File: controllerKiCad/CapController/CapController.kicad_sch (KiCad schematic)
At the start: 16 parts

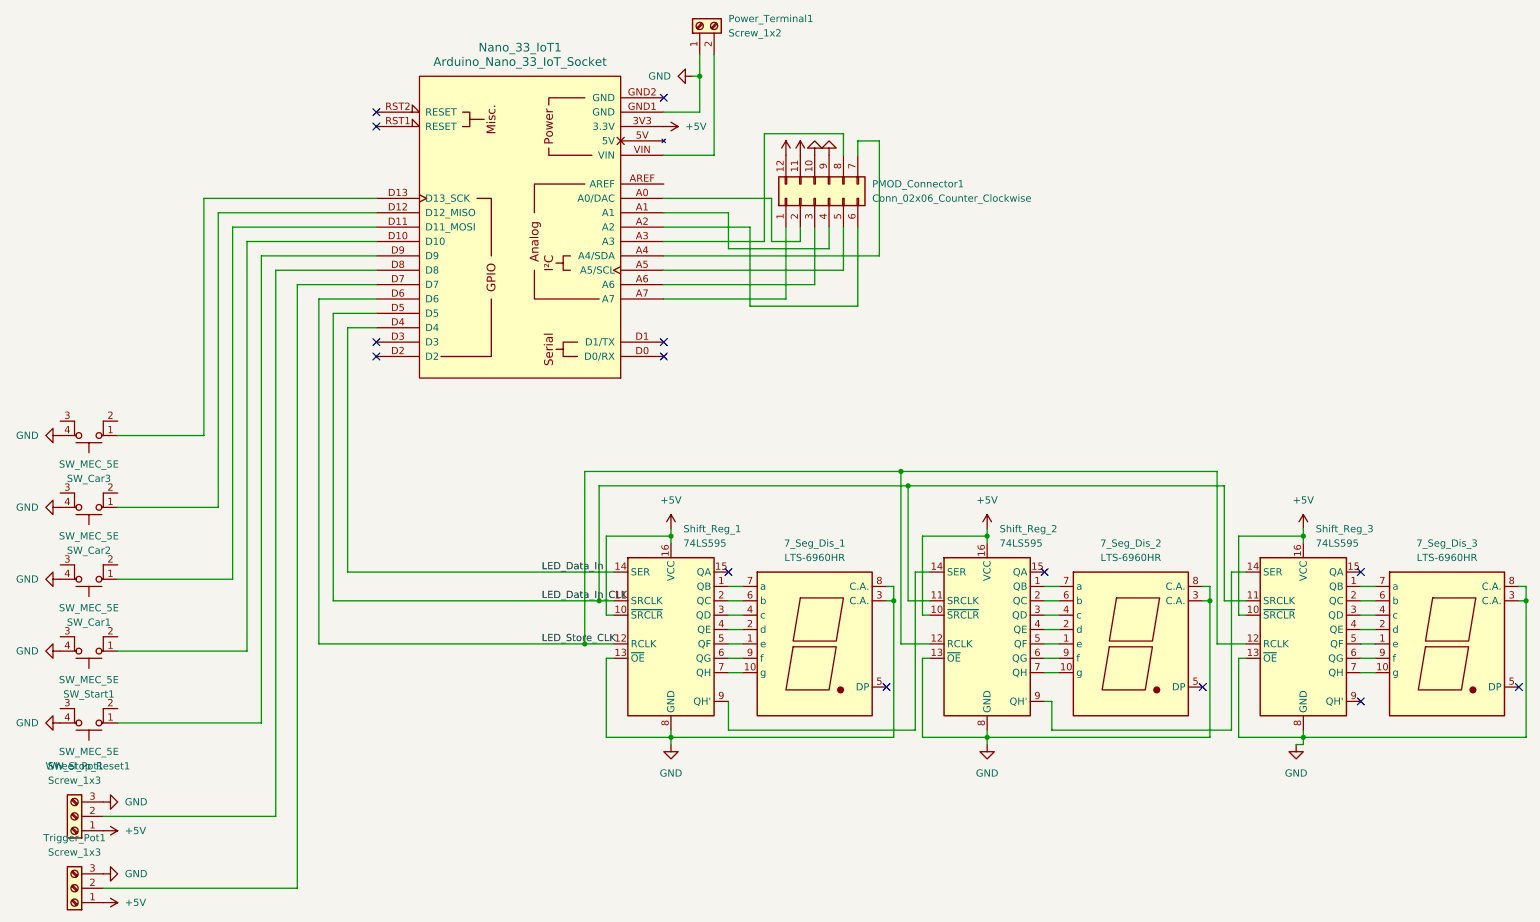
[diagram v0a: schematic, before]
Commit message: updated controller kicad files
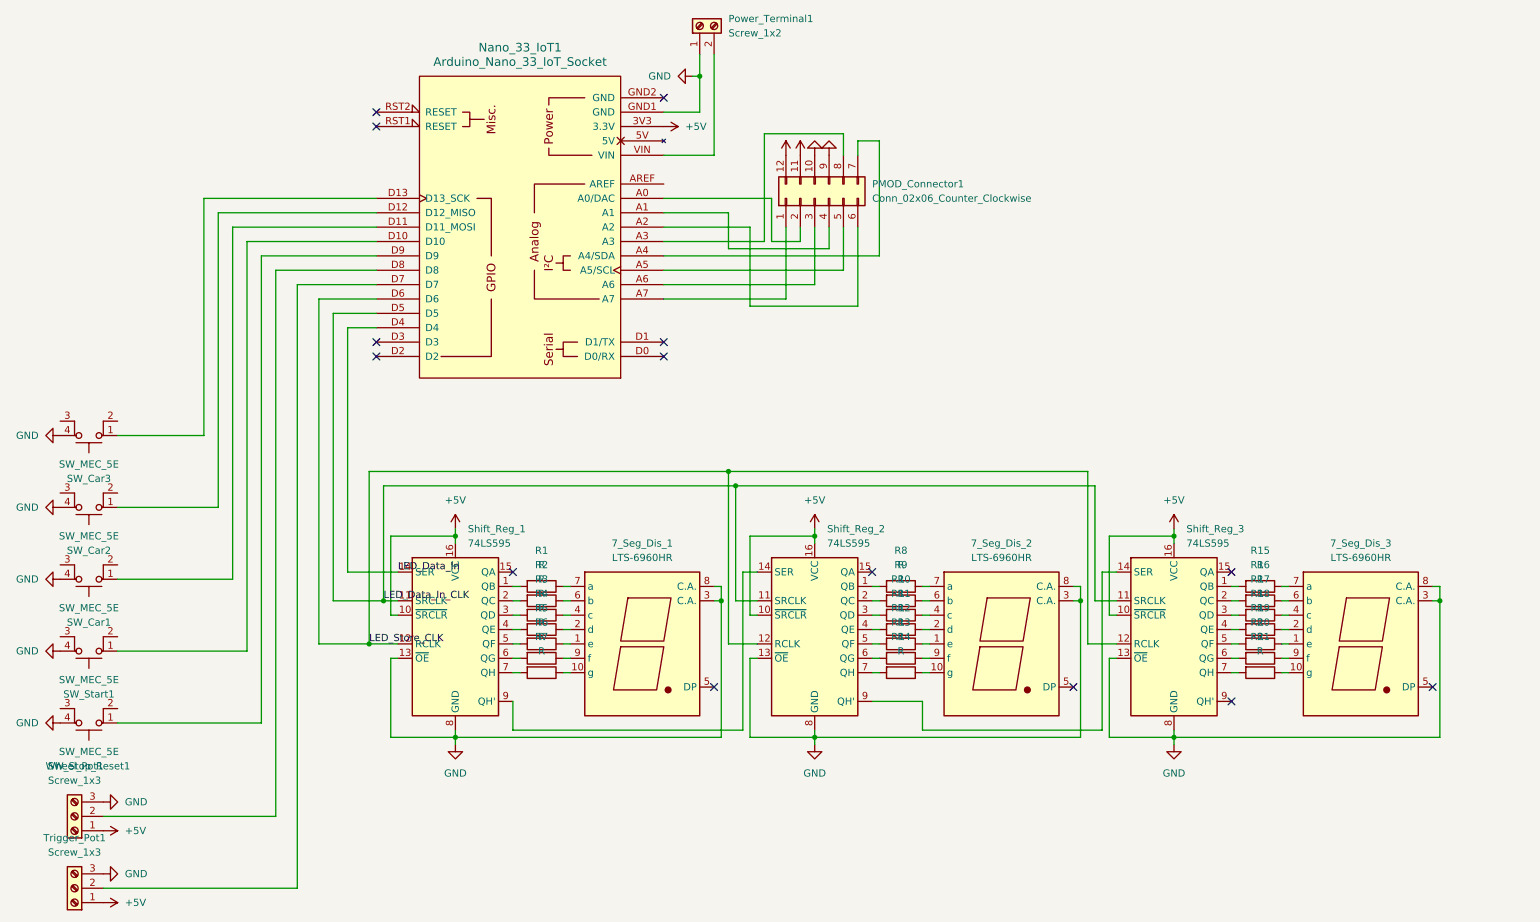
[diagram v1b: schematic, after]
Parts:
- added R1, R10, R11, R12, R13, R14, R15, R16, R17, R18, R19, R2, R20, R21, R3, R4, R5, R6, R7, R8, R9: R, Resistor_THT:R_Axial_DIN0309_L9.0mm_D3.2mm_P12.70mm_Horizontal, symbol Device:R
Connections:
- net at 7_Seg_Dis_3.1 (e): now also R19.1; no longer Shift_Reg_3.5 (QF)
- net at 7_Seg_Dis_3.10 (g): now also R21.1; no longer Shift_Reg_3.7 (QH)
- net at 7_Seg_Dis_3.2 (d): now also R18.1; no longer Shift_Reg_3.4 (QE)
- net at 7_Seg_Dis_3.4 (c): now also R17.1; no longer Shift_Reg_3.3 (QD)
- net at 7_Seg_Dis_3.6 (b): now also R16.1; no longer Shift_Reg_3.2 (QC)
- net at 7_Seg_Dis_3.7 (a): now also R15.1; no longer Shift_Reg_3.1 (QB)
- net at 7_Seg_Dis_3.9 (f): now also R20.1; no longer Shift_Reg_3.6 (QG)
- net at 7_Seg_Dis_2.1 (e): now also R12.1; no longer Shift_Reg_2.5 (QF)
- net at 7_Seg_Dis_2.10 (g): now also R14.1; no longer Shift_Reg_2.7 (QH)
- net at 7_Seg_Dis_2.2 (d): now also R11.1; no longer Shift_Reg_2.4 (QE)
- net at 7_Seg_Dis_2.4 (c): now also R10.1; no longer Shift_Reg_2.3 (QD)
- net at 7_Seg_Dis_2.6 (b): now also R9.1; no longer Shift_Reg_2.2 (QC)
- net at 7_Seg_Dis_2.7 (a): now also R8.1; no longer Shift_Reg_2.1 (QB)
- net at 7_Seg_Dis_2.9 (f): now also R13.1; no longer Shift_Reg_2.6 (QG)
- net at Shift_Reg_1.1 (QB): now also R1.2; no longer 7_Seg_Dis_1.7 (a)
- net at 7_Seg_Dis_1.6 (b): now also R2.1; no longer Shift_Reg_1.2 (QC)
- net at 7_Seg_Dis_1.4 (c): now also R3.1; no longer Shift_Reg_1.3 (QD)
- net at Shift_Reg_1.4 (QE): now also R4.2; no longer 7_Seg_Dis_1.2 (d)
- net at 7_Seg_Dis_1.1 (e): now also R5.1; no longer Shift_Reg_1.5 (QF)
- net at 7_Seg_Dis_1.9 (f): now also R6.1; no longer Shift_Reg_1.6 (QG)
- net at Shift_Reg_1.7 (QH): now also R7.2; no longer 7_Seg_Dis_1.10 (g)
- new net: R13.2, Shift_Reg_2.6 (QG)
- new net: R19.2, Shift_Reg_3.5 (QF)
- new net: R6.2, Shift_Reg_1.6 (QG)
- new net: R10.2, Shift_Reg_2.3 (QD)
- new net: R14.2, Shift_Reg_2.7 (QH)
- new net: R5.2, Shift_Reg_1.5 (QF)
- new net: R8.2, Shift_Reg_2.1 (QB)
- new net: R9.2, Shift_Reg_2.2 (QC)
- new net: R11.2, Shift_Reg_2.4 (QE)
- new net: R12.2, Shift_Reg_2.5 (QF)
- new net: R20.2, Shift_Reg_3.6 (QG)
- new net: R3.2, Shift_Reg_1.3 (QD)
- new net: R15.2, Shift_Reg_3.1 (QB)
- new net: R16.2, Shift_Reg_3.2 (QC)
- new net: R17.2, Shift_Reg_3.3 (QD)
- new net: R18.2, Shift_Reg_3.4 (QE)
- new net: R21.2, Shift_Reg_3.7 (QH)
- new net: R2.2, Shift_Reg_1.2 (QC)
- new net: 7_Seg_Dis_1.10 (g), R7.1
- new net: 7_Seg_Dis_1.2 (d), R4.1
- new net: 7_Seg_Dis_1.7 (a), R1.1
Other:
- moved on the sheet: 7_Seg_Dis_1, 7_Seg_Dis_2, 7_Seg_Dis_3, Shift_Reg_1, Shift_Reg_2, Shift_Reg_3
